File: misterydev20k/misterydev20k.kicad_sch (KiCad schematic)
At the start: 53 parts, among them J1 SWD, J2 USB_C_Receptacle_USB2.0, SW1 SW_Push, U1 SY8113BADC, U2 W25Q128JVS, U3 USBLC6-2SC6, U4 RP2040, Y1 12MHz

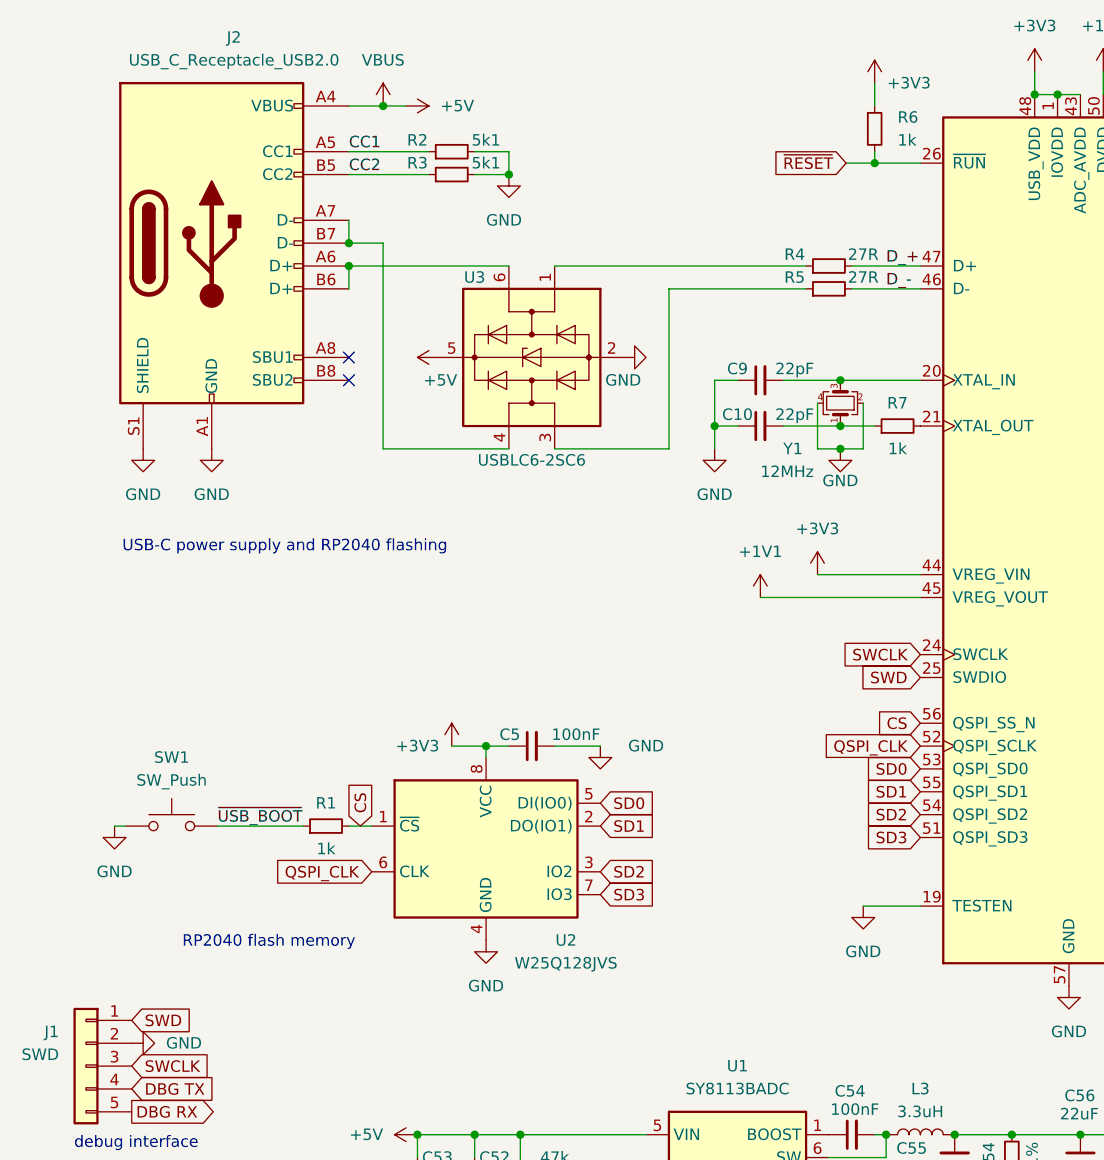
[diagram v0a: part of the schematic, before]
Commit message: Further work on the dev20k
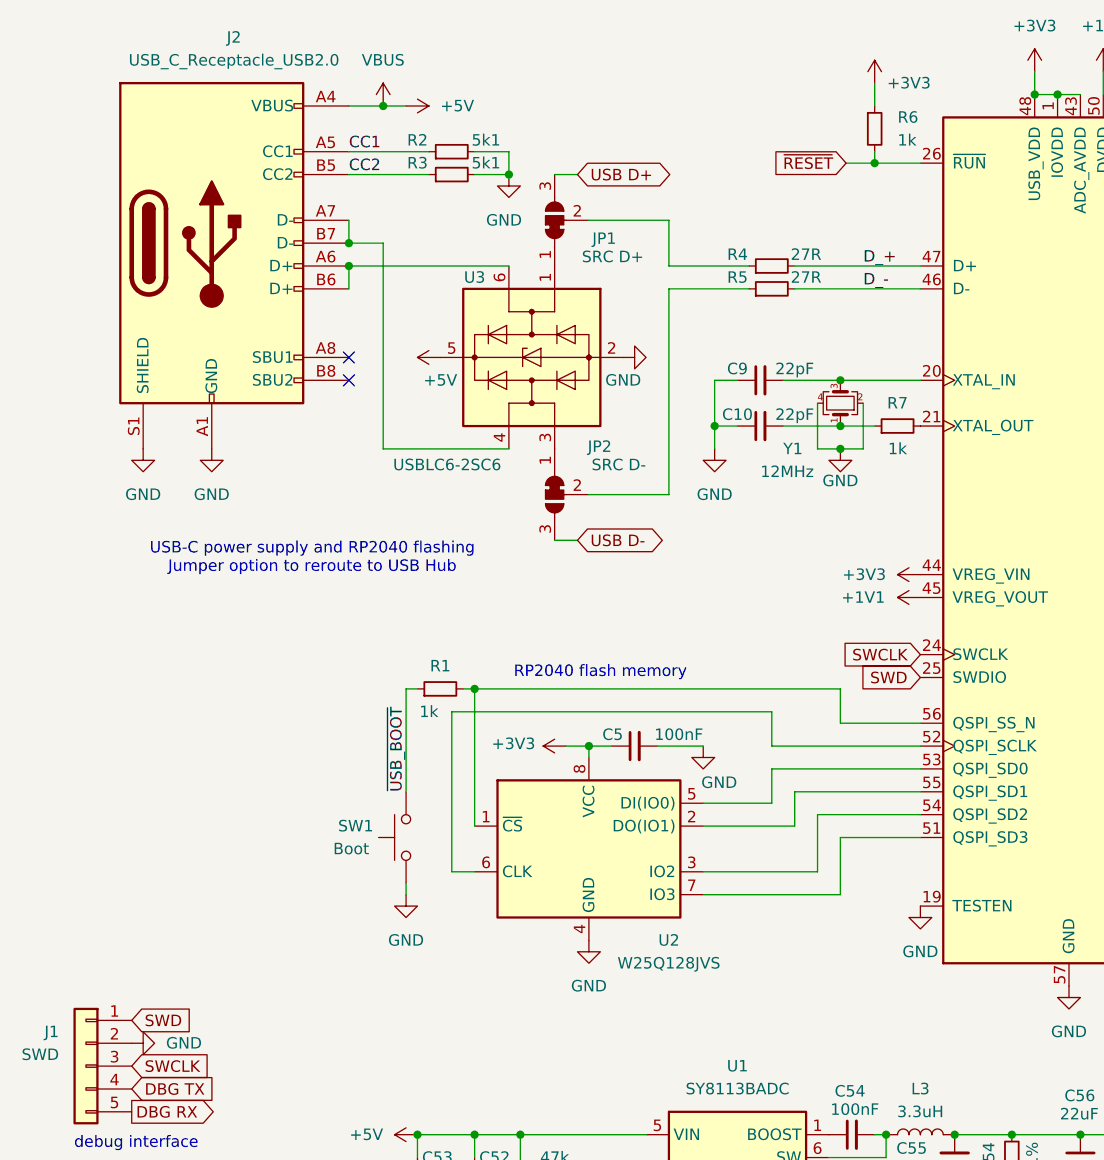
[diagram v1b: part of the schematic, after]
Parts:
- added JP1: SRC D+, Jumper:SolderJumper-3_P1.3mm_Bridged12_RoundedPad1.0x1.5mm, symbol Jumper:SolderJumper_3_Bridged12
- added JP2: SRC D-, Jumper:SolderJumper-3_P1.3mm_Bridged12_RoundedPad1.0x1.5mm, symbol Jumper:SolderJumper_3_Bridged12
- SW1: value SW_Push -> Boot
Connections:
- net USB D+: now also JP1.3 (B)
- net USB D-: now also JP2.3 (B)
- net at U3.1 (I/O1): now also JP1.1 (A); no longer R4.1
- net at U3.3 (I/O2): now also JP2.1 (A); no longer R5.1
- net CS: no longer names the net of R1.2, U2.1 (~{CS}), U4.56 (QSPI_SS_N)
- net QSPI_CLK: no longer names the net of U2.6 (CLK), U4.52 (QSPI_SCLK)
- net SD0: no longer names the net of U2.5 (DI(IO0)), U4.53 (QSPI_SD0)
- net SD1: no longer names the net of U2.2 (DO(IO1)), U4.55 (QSPI_SD1)
- net SD2: no longer names the net of U2.3 (IO2), U4.54 (QSPI_SD2)
- net SD3: no longer names the net of U2.7 (IO3), U4.51 (QSPI_SD3)
- new net: JP2.2 (C), R5.1
- new net: JP1.2 (C), R4.1
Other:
- note added: "USB-C power supply and RP2040 flashing Jumper option to reroute to USB Hub"
- note removed: "USB-C power supply and RP2040 flashing"
- moved on the sheet: C5, R1, R4, R5, SW1, U2
